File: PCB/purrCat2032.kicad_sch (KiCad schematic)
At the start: 18 parts, among them M1 Motor_DC_ALT, Q1 Q_NMOS_GSD, U1 MSP430FR2110/MSP430FR2111

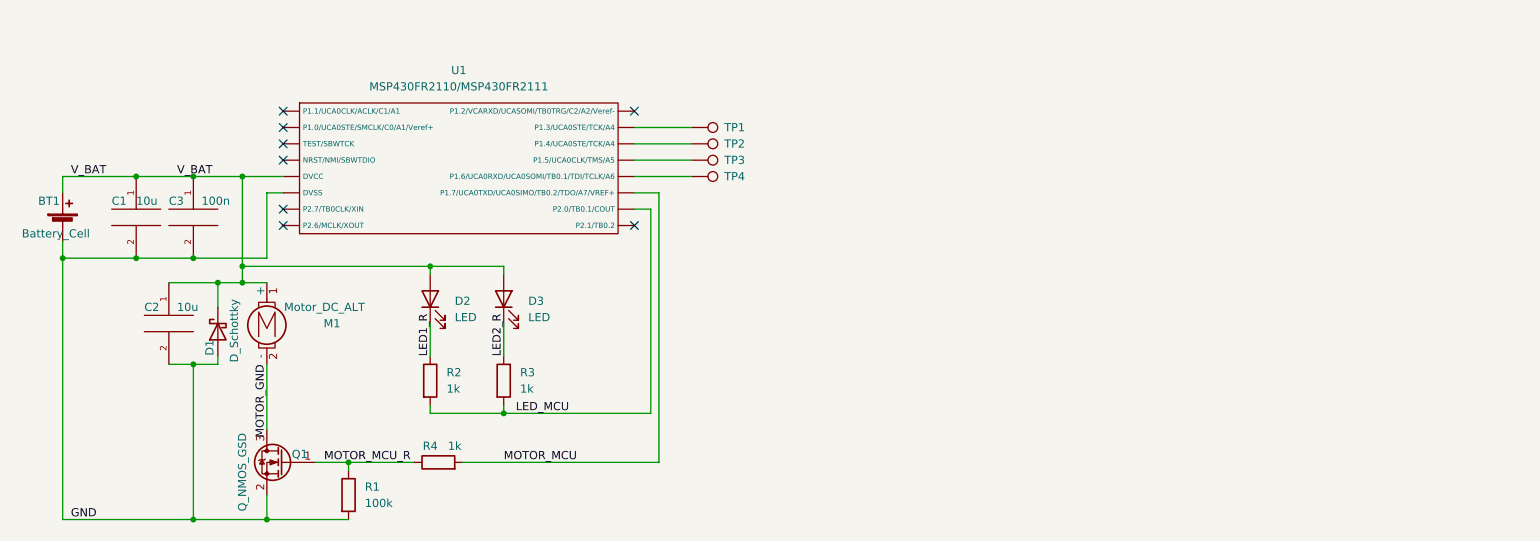
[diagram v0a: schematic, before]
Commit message: new design!
+all sort of junk kicad files - will cleanup later
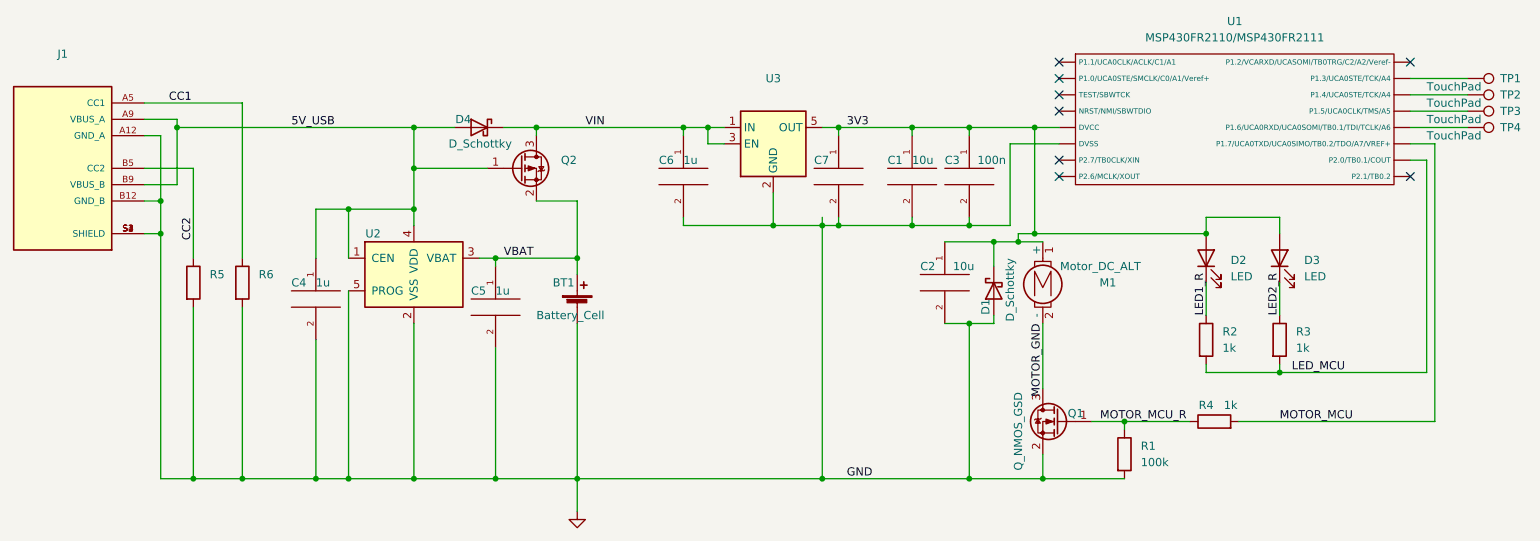
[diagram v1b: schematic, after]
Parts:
- added C4, C5, C6: 1u, Capacitor_SMD:C_0805_2012Metric, symbol pspice:CAP
- added C7: (no value), Capacitor_SMD:C_0805_2012Metric, symbol pspice:CAP
- added D4: D_Schottky, Diode_SMD:D_0603_1608Metric, symbol Device:D_Schottky
- added J1: (no value), symbol USB4135-GF-A_REVA:USB4135-GF-A_REVA
- added Q2: (no value), symbol Device:Q_PMOS_GSD
- added R5, R6: (no value), symbol Device:R
- added U2: (no value), symbol Battery_Management:MCP73811T-420I-OT
- added U3: (no value), symbol Regulator_Linear:TPS7A0533PDBV
- TP1, TP2, TP3, TP4: value (none) -> TouchPad
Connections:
- net GND: now also C4.2, C5.2, C6.2, C7.2, J1.A12 (GND_A), J1.B12 (GND_B), J1.S1 (SHIELD), J1.S2 (SHIELD), J1.S3 (SHIELD), J1.S4 (SHIELD), R5.2, R6.2, U2.2 (VSS), U2.5 (PROG), U3.2 (GND)
- net V_BAT renamed 3V3
- net 3V3: now also C7.1, U3.5 (OUT); no longer BT1.1 (+)
- new net 5V_USB: C4.1, D4.2 (A), J1.A9 (VBUS_A), J1.B9 (VBUS_B), Q2.1 (G), U2.1 (CEN), U2.4 (VDD)
- new net CC1: J1.A5 (CC1), R6.1
- new net CC2: J1.B5 (CC2), R5.1
- new net VBAT: BT1.1 (+), C5.1, Q2.2 (S), U2.3 (VBAT)
- new net VIN: C6.1, D4.1 (K), Q2.3 (D), U3.1 (IN), U3.3 (EN)
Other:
- moved on the sheet: BT1, C1, C2, C3, D1, D2, D3, M1, Q1, R1, R2, R3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
